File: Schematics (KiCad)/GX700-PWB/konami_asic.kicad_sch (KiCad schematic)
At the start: 57 parts

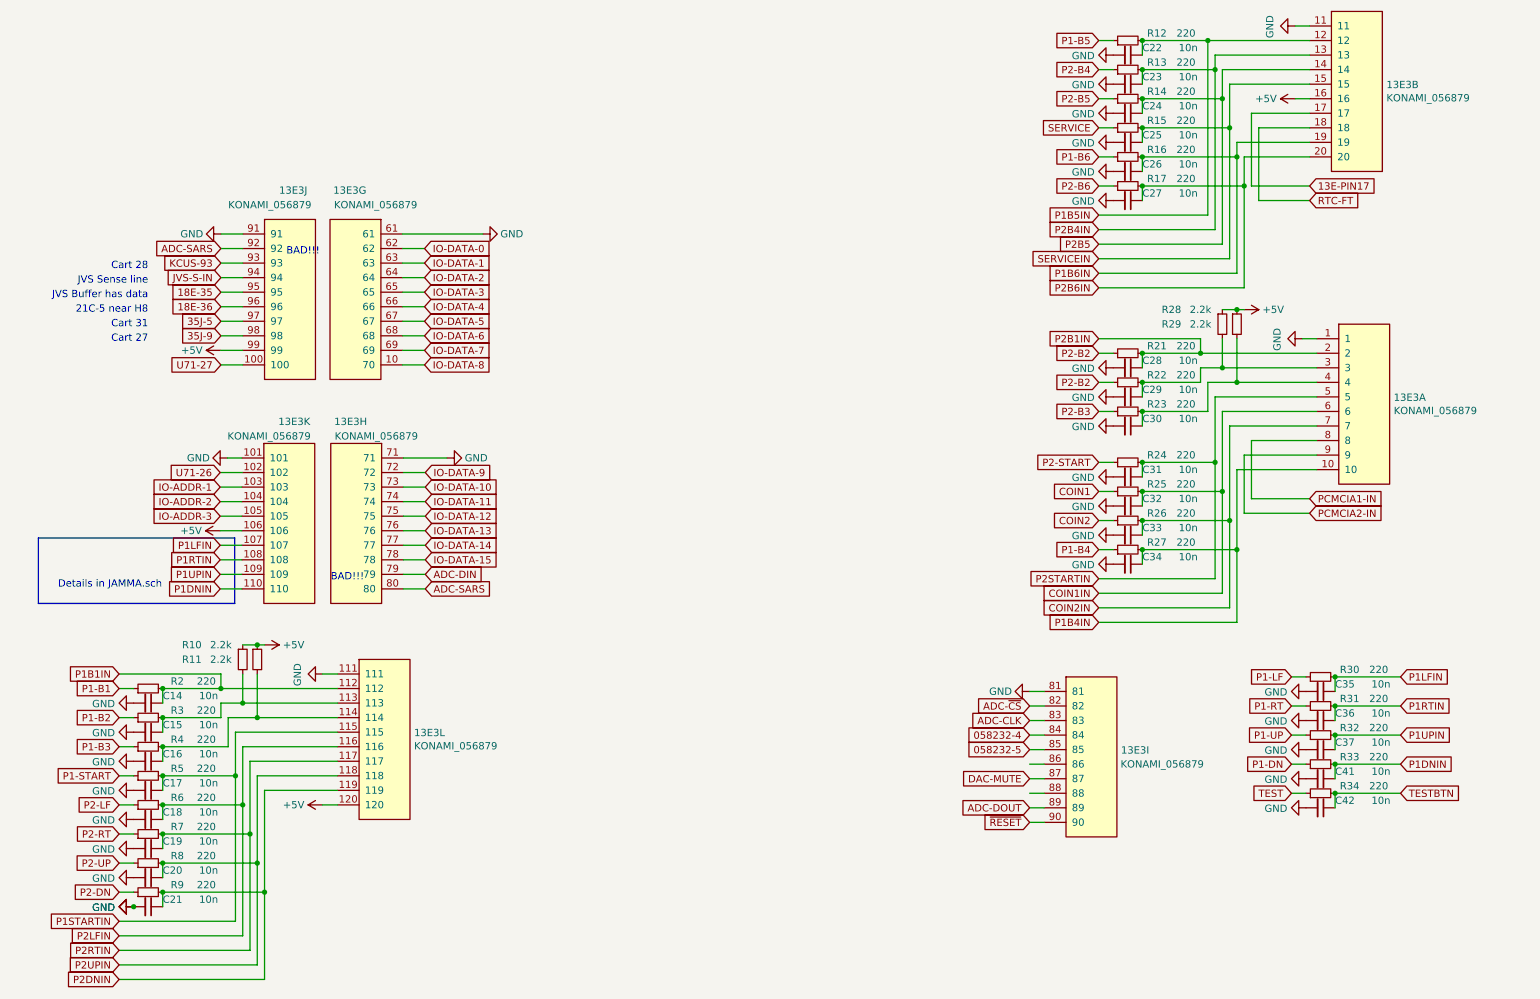
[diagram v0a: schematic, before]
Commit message: General Fixes
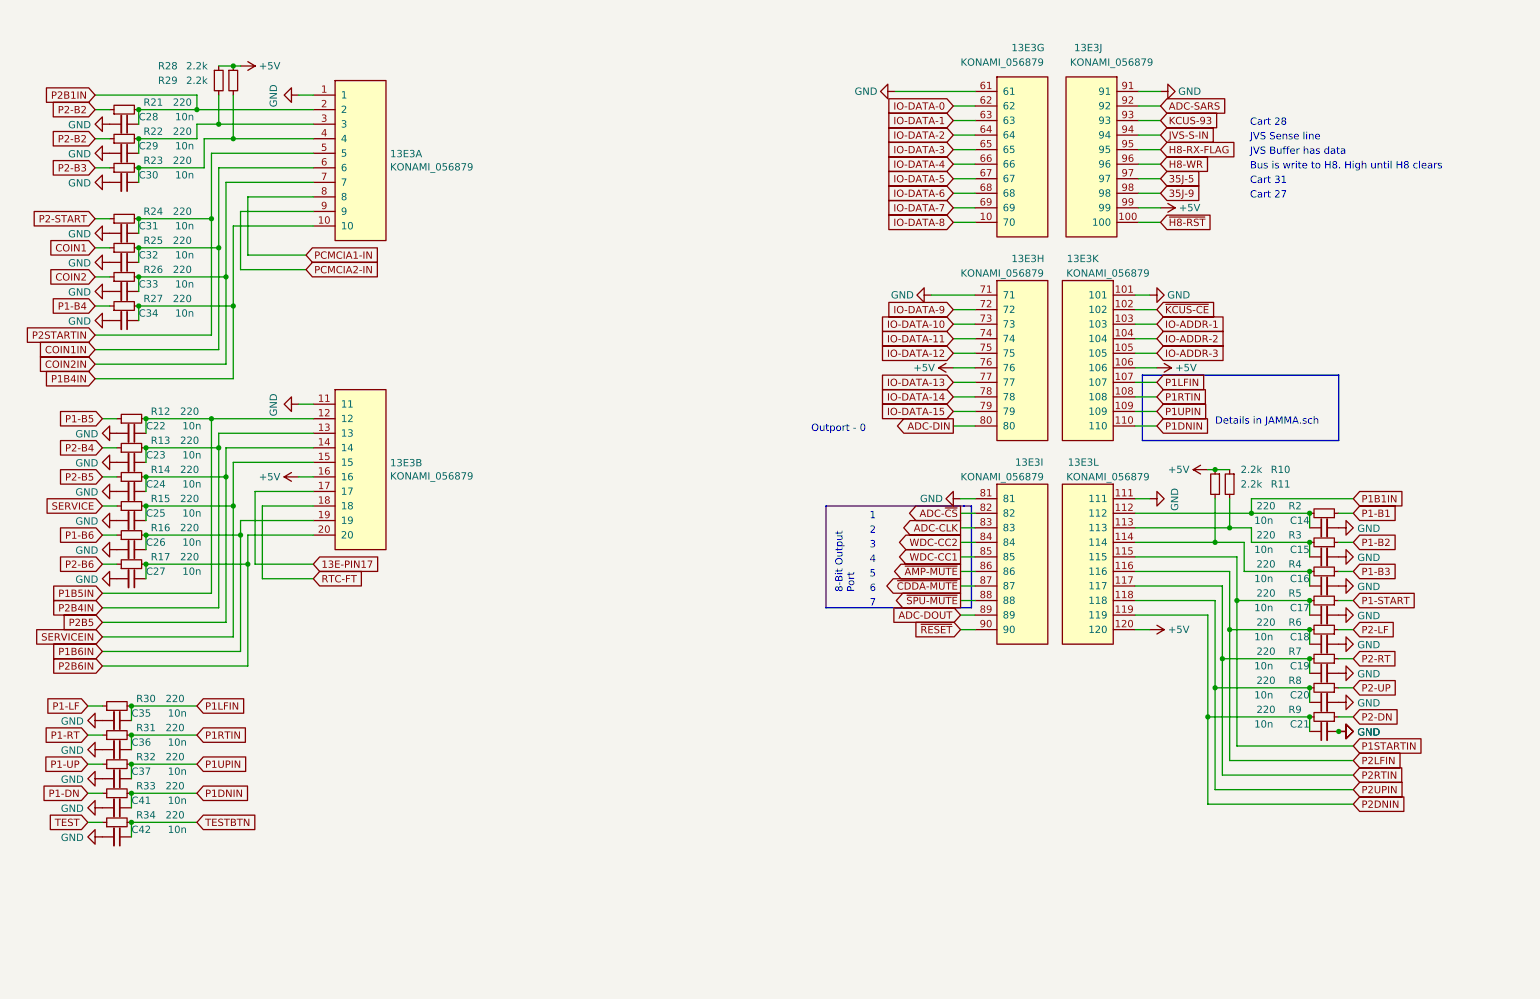
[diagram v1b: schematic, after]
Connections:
- net +5V: now also 13E3.76
- net ADC-DIN: now also 13E3.80; no longer 13E3.79
- net ADC-SARS: no longer 13E3.80
- net IO-DATA-13: now also 13E3.77; no longer 13E3.76
- net IO-DATA-14: now also 13E3.78; no longer 13E3.77
- net IO-DATA-15: now also 13E3.79; no longer 13E3.78
- net ~{AMP-MUTE}: now reaches 13E3.86
- net ~{SPU-MUTE}: now reaches 13E3.88
- net 058232-4 renamed WDC-CC2
- net 058232-5 renamed WDC-CC1
- net 18E-35 renamed H8-RX-FLAG
- net 18E-36 renamed H8-WR
- net DAC-MUTE renamed ~{CDDA-MUTE}
- net U71-26 renamed ~{KCUS-CE}
- net U71-27 renamed ~{H8-RST}
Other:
- note added: "1"
- note added: "2"
- note added: "3"
- note added: "4"
- note added: "5"
- note added: "6"
- note added: "7"
- note added: "8-Bit Output Port"
- note added: "Bus is write to H8. High until H8 clears"
- note added: "Outport - 0"
- note removed: "21C-5 near H8"
- note removed: "BAD!!!"
- moved on the sheet: 13E3A, 13E3B, 13E3G, 13E3H, 13E3I, 13E3J, 13E3K, 13E3L, C14, C15, C16, C17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
